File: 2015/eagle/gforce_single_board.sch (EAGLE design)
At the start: 5 parts, among them U1 ATMEGA328P_PDIP

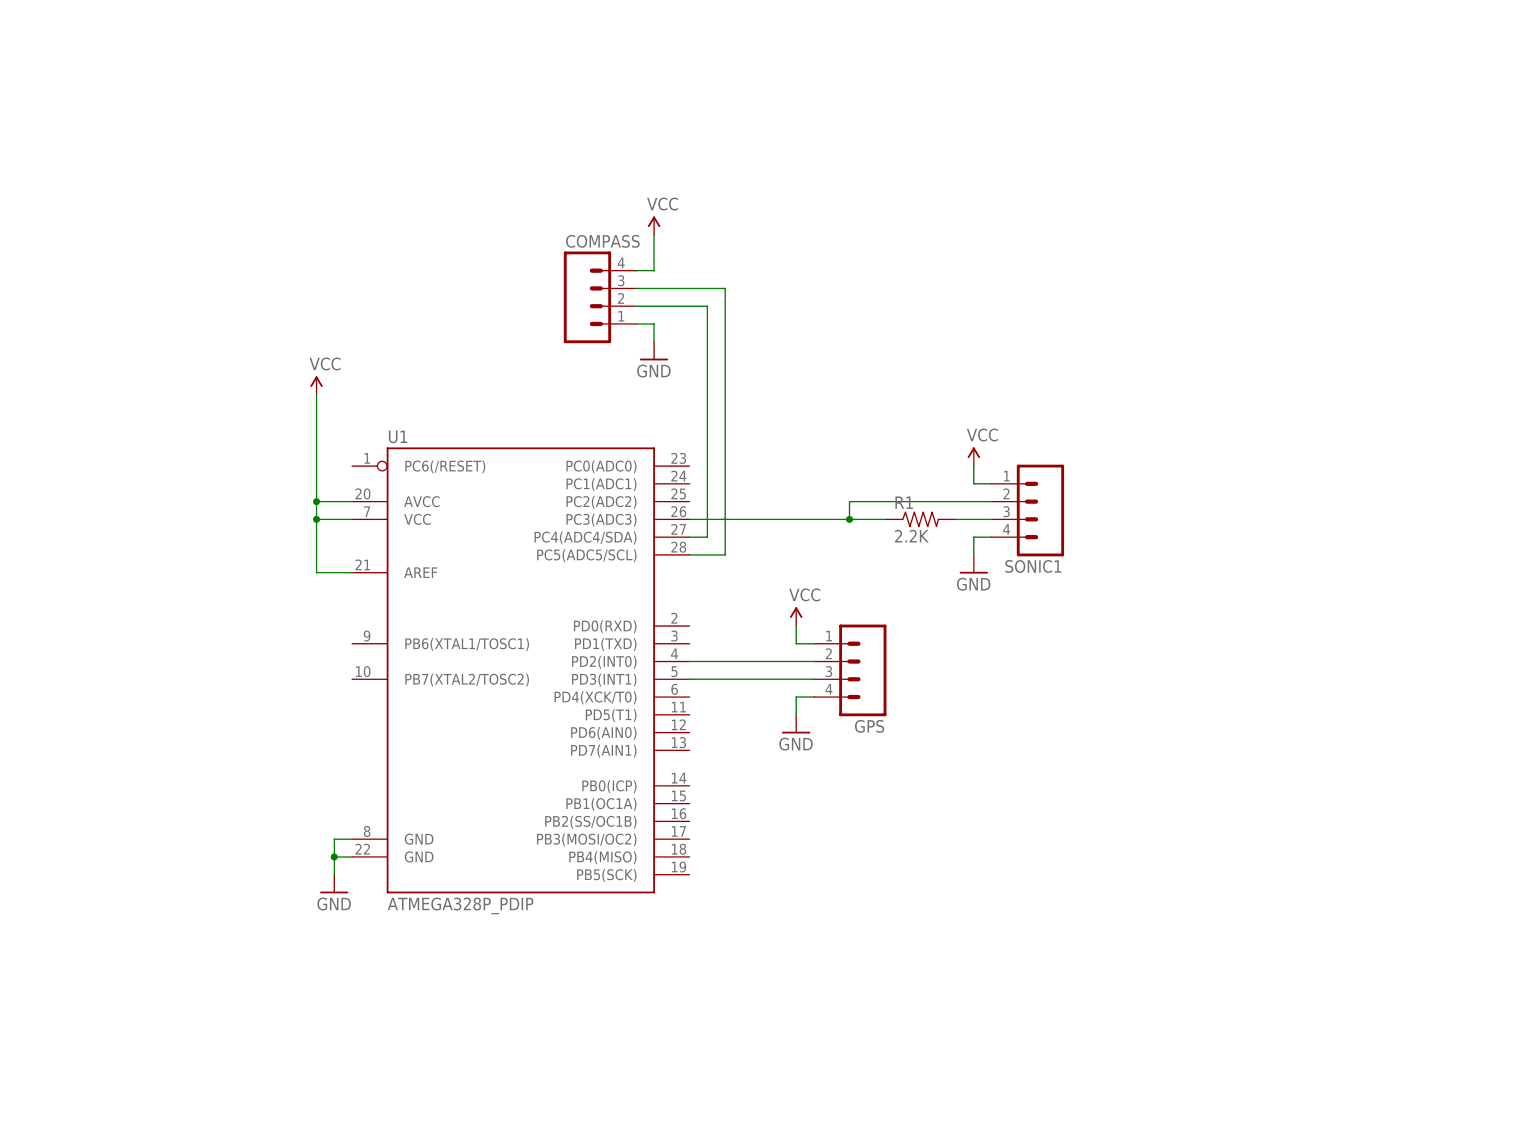
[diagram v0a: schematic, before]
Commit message: save
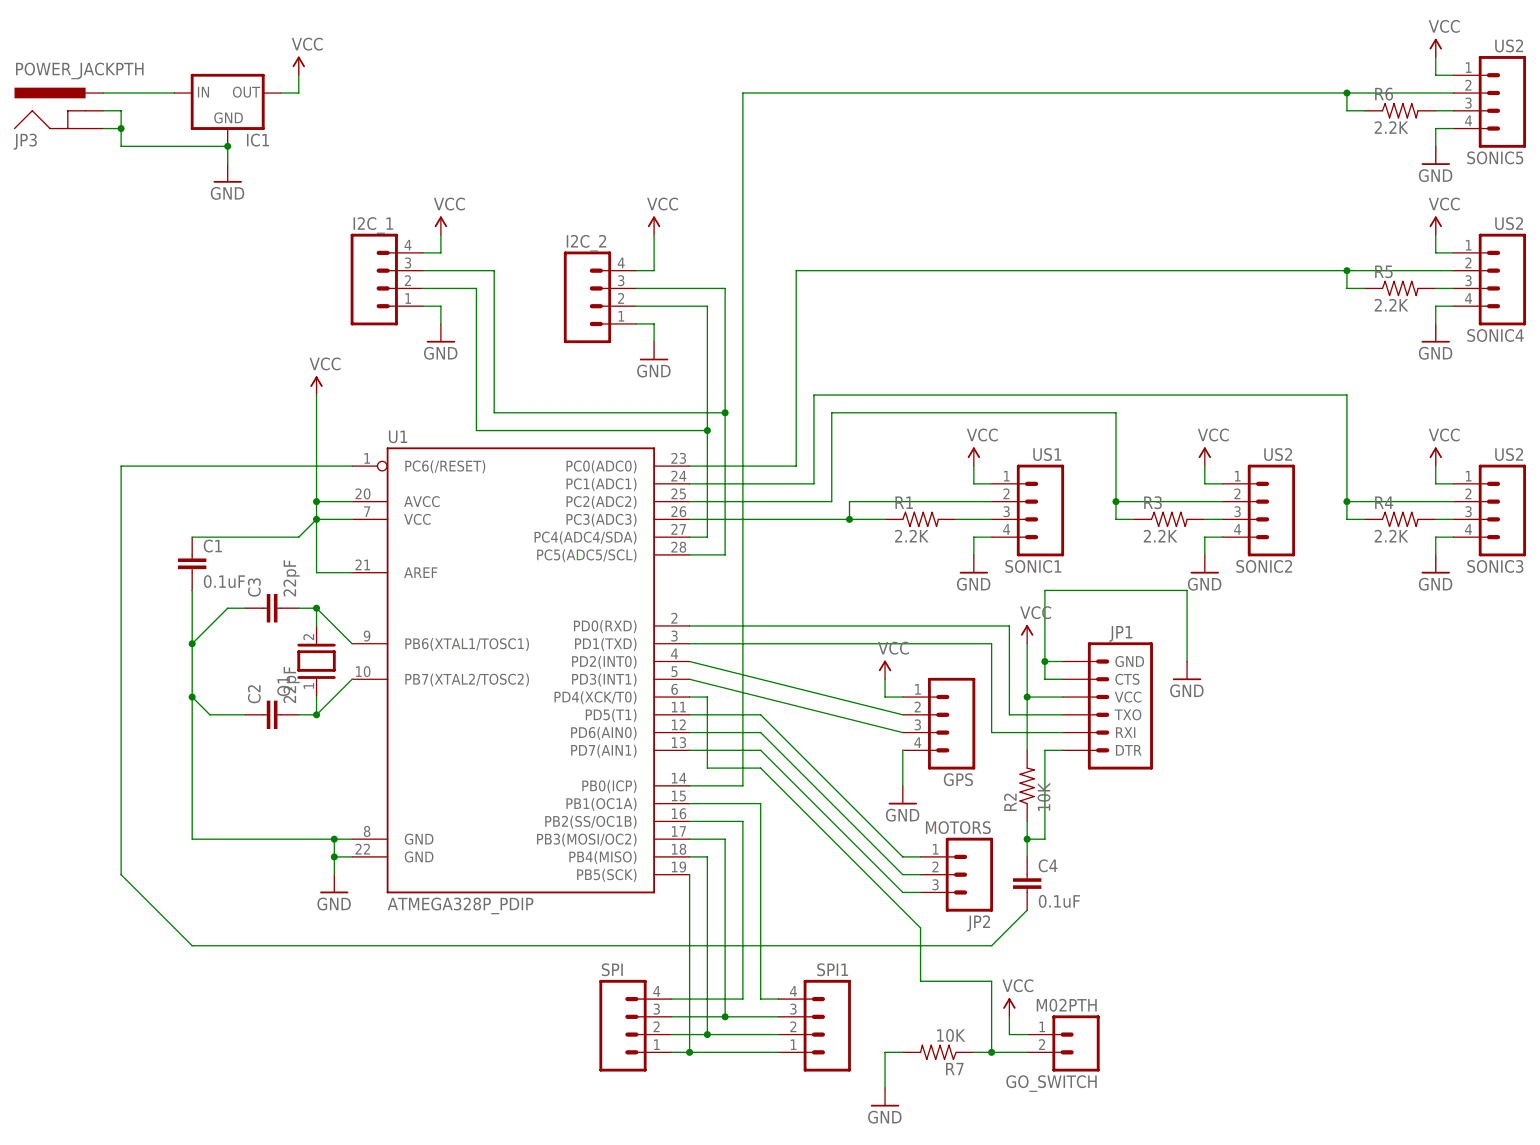
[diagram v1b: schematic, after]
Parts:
- added C1, C4: 0.1uF, SparkFun-Passives:CAPPTH
- added C2, C3: 22pF, SparkFun-Passives:CAPPTH
- added GO_SWITCH: M02PTH, SparkFun-Connectors:M02PTH
- added I2C_1, SPI, SPI1: (no value), SparkFun-Connectors:M04PTH
- added IC1: (no value), SparkFun-PowerIC:V_REG_78XX-TO-220
- added JP1: (no value), SparkFun-Connectors:ARDUINO_SERIAL_PROGRAMPTH
- added JP2: MOTORS, SparkFun-Connectors:M03PTH
- added JP3: POWER_JACKPTH, SparkFun-Connectors:POWER_JACKPTH
- added Q1: (no value), special:XTAL/S
- added R2, R7: 10K, SparkFun-Resistors:RESISTORPTH-1/4W
- added R3, R4, R5, R6: 2.2K, SparkFun-Resistors:RESISTORPTH-1/4W
- added SONIC2, SONIC3, SONIC4, SONIC5: US2, SparkFun-Connectors:M04PTH
- SONIC1: value (none) -> US1
- renumbered COMPASS to I2C_2
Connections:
- new net MISO: SPI.2, SPI1.2, U1.PB4(MISO)
- new net MOSI: SPI.3, SPI1.3, U1.PB3(MOSI/OC2)
- new net N$10: C4.1, JP1.DTR, R2.1
- new net N$11: R3.2, SONIC2.3
- new net N$12: R3.1, SONIC2.2, U1.PC2(ADC2)
- new net N$13: JP2.1, U1.PD5(T1)
- new net N$14: R4.2, SONIC3.3
- new net N$15: R4.1, SONIC3.2, U1.PC1(ADC1)
- new net N$16: R6.2, SONIC5.3
- new net N$17: R6.1, SONIC5.2, U1.PB0(ICP)
- new net N$18: JP2.2, U1.PD6(AIN0)
- new net N$19: R5.2, SONIC4.3
- new net N$20: R5.1, SONIC4.2, U1.PC0(ADC0)
- new net N$21: JP2.3, U1.PD7(AIN1)
- new net N$22: SPI.4, U1.PB2(SS/OC1B)
- new net N$23: SPI1.4, U1.PB1(OC1A)
- new net N$26: GO_SWITCH.2, R7.1, U1.PD4(XCK/T0)
- new net N$27: IC1.IN, JP3.PWR
- new net N$5: C3.2, Q1.2, U1.PB6(XTAL1/TOSC1)
- new net N$6: C2.2, Q1.1, U1.PB7(XTAL2/TOSC2)
- new net N$7: JP1.RXI, U1.PD1(TXD)
- new net N$8: JP1.TXO, U1.PD0(RXD)
- new net N$9: C4.2, U1.PC6(/RESET)
- new net SCK: SPI.1, SPI1.1, U1.PB5(SCK)
- net GND: now also C1.2, C2.1, C3.1, I2C_1.1, IC1.GND, JP1.CTS, JP1.GND, JP3.GND, JP3.GNDBREAK, R7.2, SONIC2.4, SONIC3.4, SONIC4.4, SONIC5.4
- net N$1: now also I2C_1.2
- net N$2: now also I2C_1.3
- net VCC: now also C1.1, GO_SWITCH.1, I2C_1.4, IC1.OUT, JP1.VCC, R2.2, SONIC2.1, SONIC3.1, SONIC4.1, SONIC5.1
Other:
- moved on the sheet: GPS
